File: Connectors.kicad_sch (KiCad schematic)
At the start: 11 parts, among them J1 MAIN, J2 PRG CONN, U3 TJA1050T/CM,118

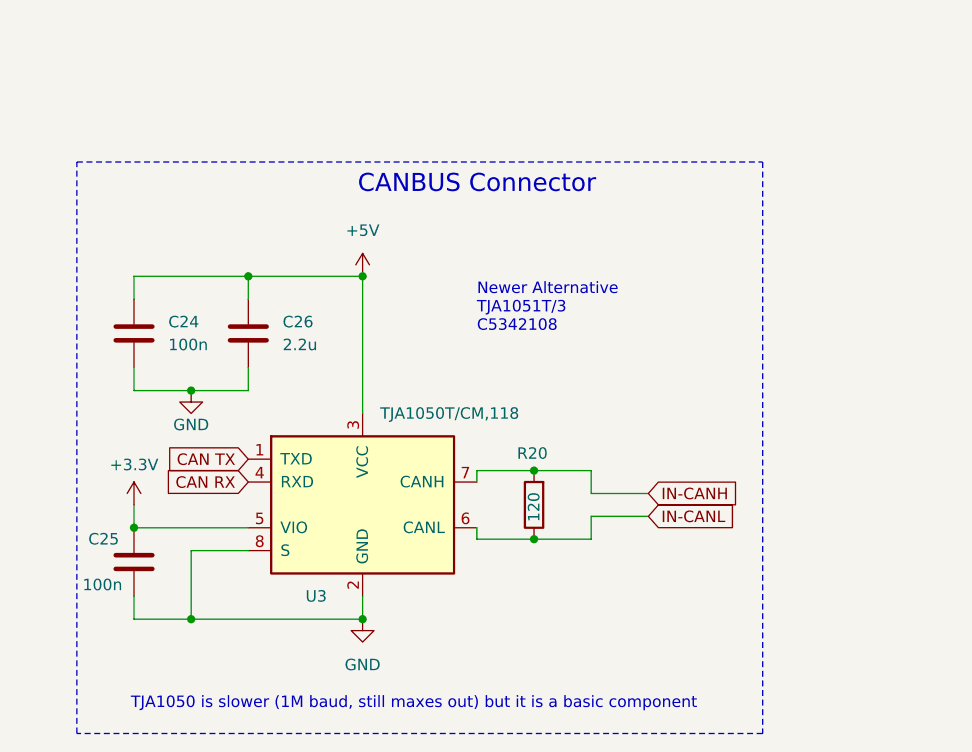
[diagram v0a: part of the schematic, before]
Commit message: modular
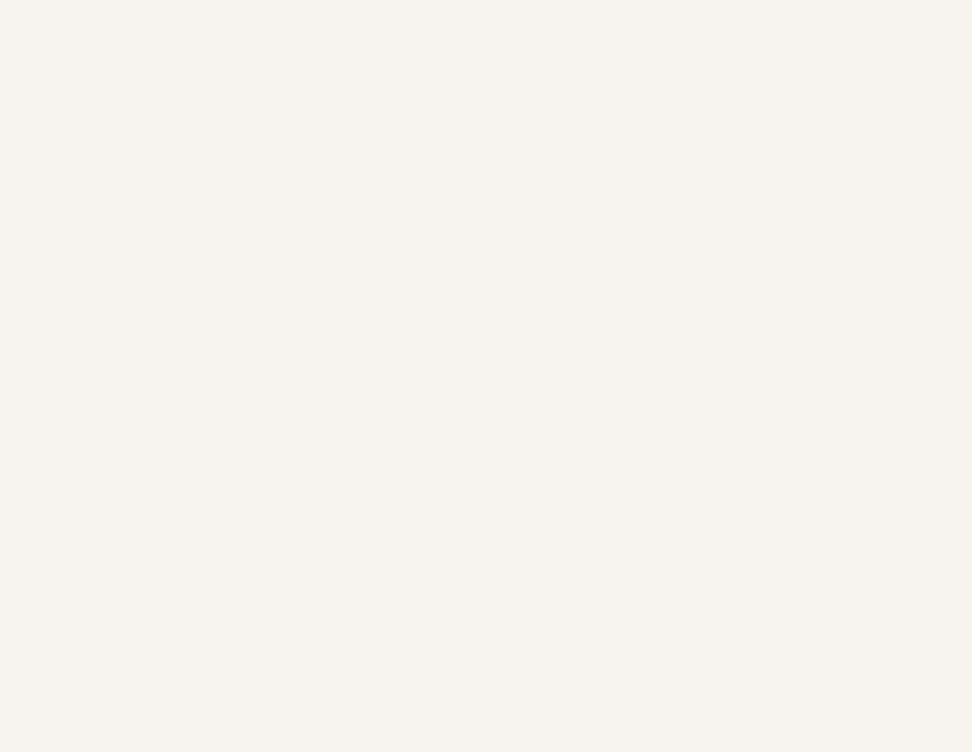
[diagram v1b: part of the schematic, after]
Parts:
- removed C24, C25: 100n, Capacitor_SMD:C_0603_1608Metric, symbol Device:C
- removed C26: 2.2u, Capacitor_SMD:C_0603_1608Metric, symbol Device:C
- removed R20: 120, Resistor_SMD:R_0603_1608Metric, symbol Device:R
- removed U3: TJA1050T/CM,118, Package_SO:SOIC-8_3.9x4.9mm_P1.27mm, symbol Interface_CAN_LIN:TJA1051T-3
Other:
- note removed: "CANBUS Connector"
- note removed: "Newer Alternative TJA1051T/3 C5342108"
- note removed: "TJA1050 is slower (1M baud, still maxes out) but it is a basic component"
